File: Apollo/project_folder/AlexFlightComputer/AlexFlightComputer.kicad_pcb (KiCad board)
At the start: 2 copper layers, 21 parts, among them IC1 WSEN-PADS_2511020213301 (Baro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, J1 BAT, J2 SW, J3 GPS, J4 Radio, U1 MLX90393SLW-ABA-011-RE (Magne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, U2 BMI270 (IMU)

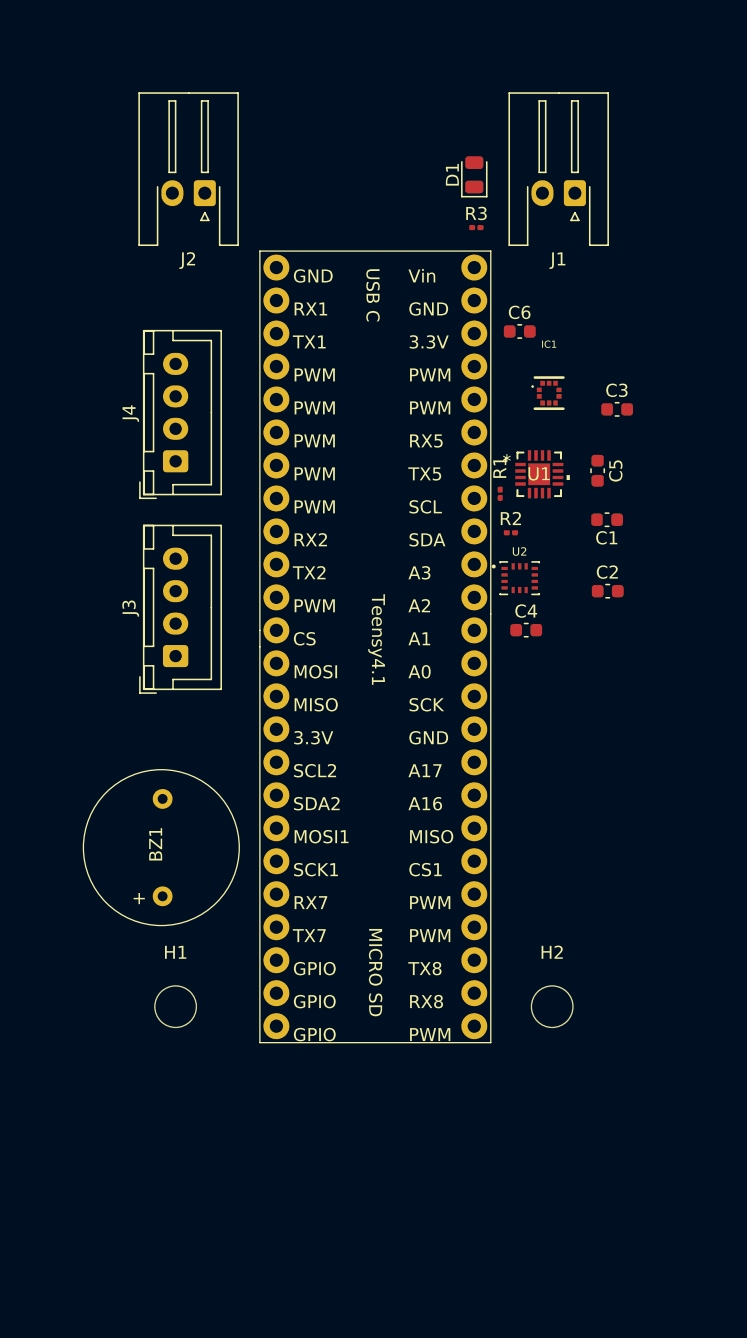
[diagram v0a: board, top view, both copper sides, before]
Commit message: Completed PCB v.1 (10/29)
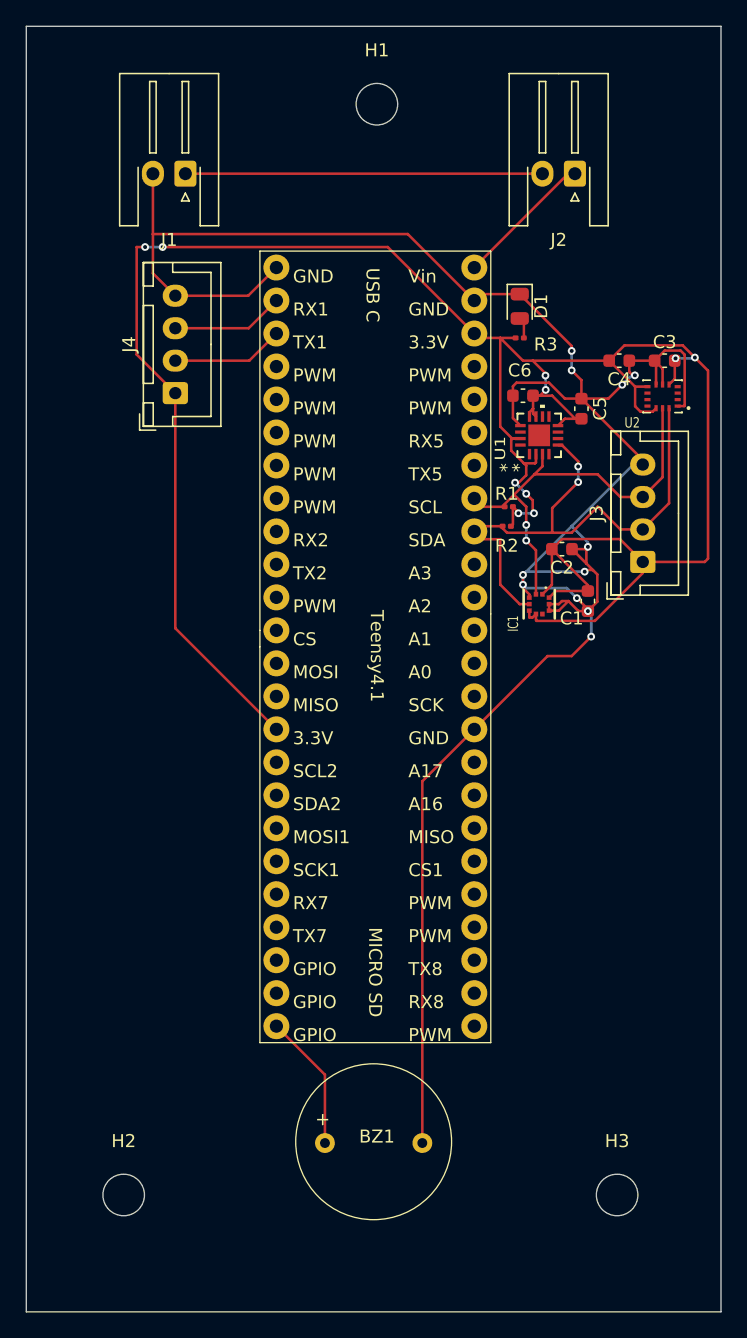
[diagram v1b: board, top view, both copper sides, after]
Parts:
- added H3: MountingHole, MountingHole:MountingHole_3.2mm_M3, F.Cu at (176.0, 116.0)
- moved H1 71.2 mm to (157.5, 32.0)
- moved J3 36.7 mm to (178.0, 67.2)
- moved H2 36.0 mm to (138.0, 116.0)
- moved J1 30.0 mm to (142.8, 37.4)
- moved J2 28.5 mm to (172.8, 37.4)
- moved BZ1 28.3 mm to (157.5, 112.0), turned to 0 degrees
- moved C4 22.0 mm to (176.2, 51.8), turned to 180 degrees
- moved U2 17.8 mm to (179.5, 54.5), turned to 180 degrees
- moved IC1 16.3 mm to (170.0, 70.5), turned to -90 degrees
- moved D1 10.7 mm to (168.5, 47.6), turned to -90 degrees
- moved R3 9.13 mm to (168.5, 50.0), turned to 180 degrees
- moved C1 6.43 mm to (173.8, 70.3), turned to 90 degrees
- moved J4 5.25 mm to (142.0, 54.2)
- moved C3 5.24 mm to (179.7, 51.8)
- moved C6 4.95 mm to (168.8, 54.4)
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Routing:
- net +3.3V: track 0.00 -> 188.1 mm, vias 0 -> 10
- net GND: track 0.00 -> 185.8 mm, vias 0 -> 11
- net /SDA: track 0.00 -> 42.5 mm, vias 0 -> 2
- net /SCL: track 0.00 -> 32.8 mm, vias 0 -> 2
- net /Batt-Sw: track 0.00 -> 27.5 mm
- net +5V: track 0.00 -> 10.7 mm
- net Net-(BZ1-+): track 0.00 -> 10.5 mm
- net /RX: track 0.00 -> 8.67 mm
- net /TX: track 0.00 -> 8.65 mm
- net Net-(D1-A): track 0.00 -> 1.63 mm
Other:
- board outline added: 53.5 x 99 mm
